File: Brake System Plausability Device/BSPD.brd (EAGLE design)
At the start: 100 x 80 mm, 47 parts, among them IC1 TLC339P, IC2 4081N, IC3 4013N, IC4 4093N, IC5 4013N, IC6 4069N, X1 ERR_STATE_OUT

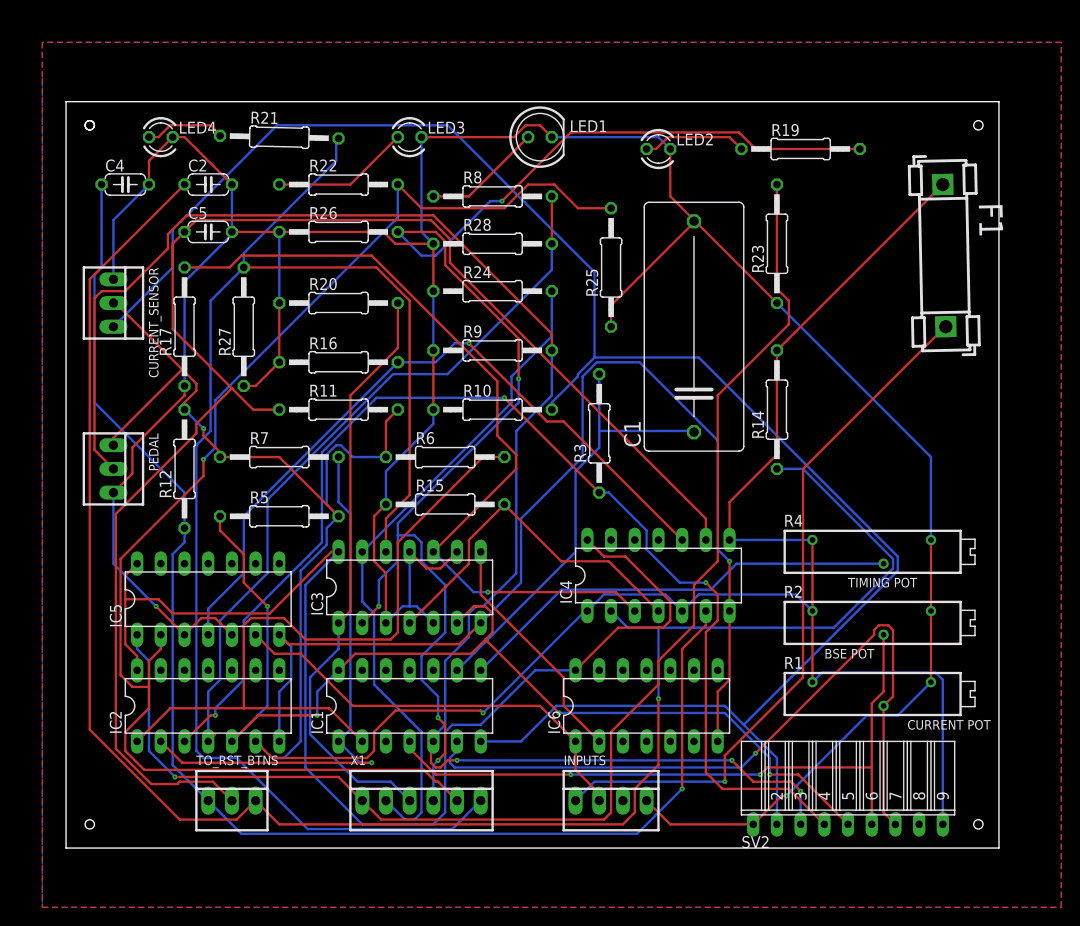
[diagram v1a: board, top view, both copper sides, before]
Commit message: PCB Designs
Rev C
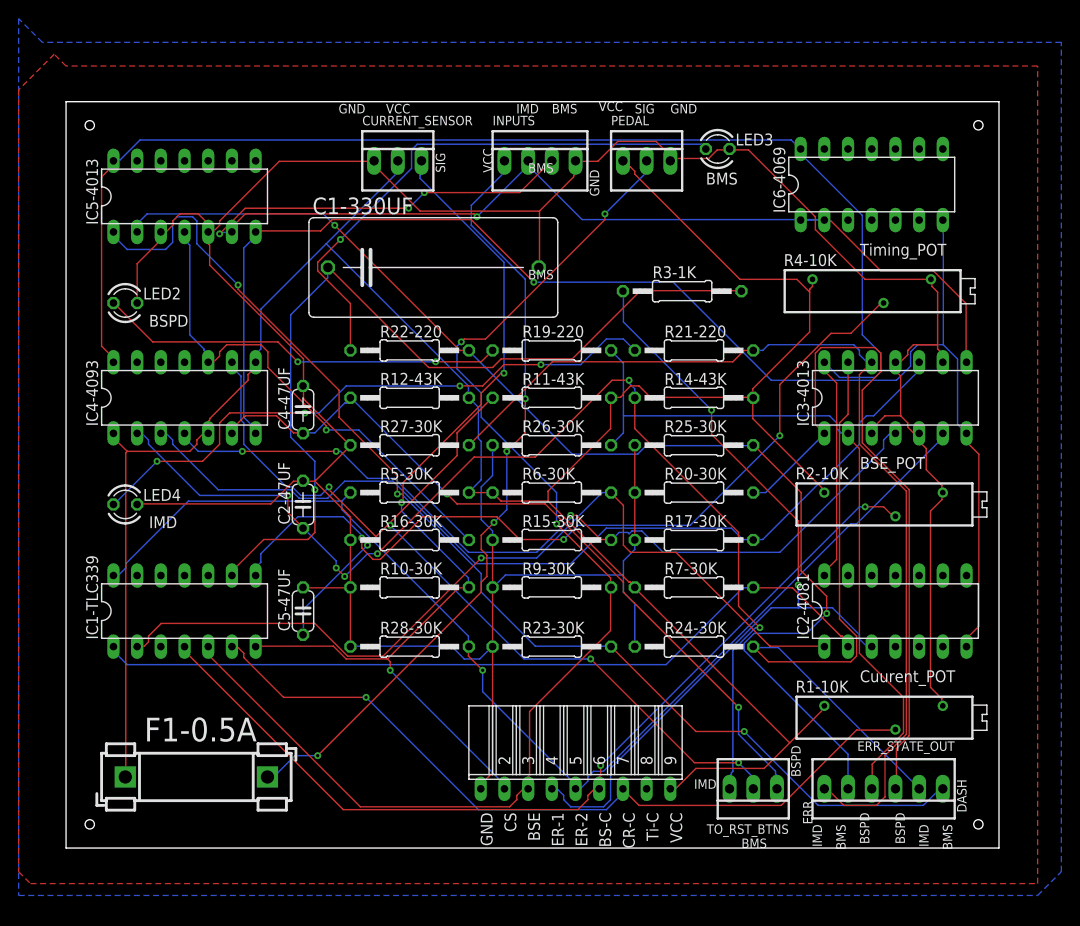
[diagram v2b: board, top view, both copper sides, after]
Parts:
- removed C1: 330u, rcl:C225-108X268
- removed C2, C4, C5: 47uF, rcl:C050-024X044
- removed F1: FUSEBLANK_5X20MM, fuse:FUSE_HOLDER_5X20MM
- removed IC1: TLC339P, linear:DIL14
- removed IC2: 4081N, 40xx:DIL14
- removed IC3, IC5: 4013N, 40xx:DIL14
- removed IC4: 4093N, 40xx:DIL14
- removed IC6: 4069N, 40xx:DIL14
- removed LED1: (no value), led:LED5MM
- removed R1, R2, R4: (no value), rcl:RTRIM3006P
- removed R10, R15, R16, R17, R20, R23, R24, R25, R26, R27, R28, R5, R6, R7, R9: 30k, rcl:0207/12
- removed R11, R12, R14: 43k, rcl:0207/12
- removed R19, R21, R22, R8: 220, rcl:0207/12
- removed R3: 1k, rcl:0207/12
- removed SV2: (no value), con-lsta:FE09W
- removed X1: ERR_STATE_OUT, con-molex:22-23-2061
- added C1-330UF: 330u, rcl:C225-108X268
- added C2-47UF, C4-47UF, C5-47UF: 47uF, rcl:C050-024X044
- added ERR_STATE_OUT: ERR_STATE_OUT, con-molex:22-23-2061
- added F1-0.5A: FUSEBLANK_5X20MM, fuse:FUSE_HOLDER_5X20MM
- added GND: (no value), con-lsta:FE09W
- added IC1-TLC339: TLC339P, linear:DIL14
- added IC2-4081: 4081N, 40xx:DIL14
- added IC3-4013, IC5-4013: 4013N, 40xx:DIL14
- added IC4-4093: 4093N, 40xx:DIL14
- added IC6-4069: 4069N, 40xx:DIL14
- added R1-10K, R2-10K, R4-10K: (no value), rcl:RTRIM3006P
- added R10-30K, R15-30K, R16-30K, R17-30K, R20-30K, R23-30K, R24-30K, R25-30K, R26-30K, R27-30K, R28-30K, R5-30K, R6-30K, R7-30K, R9-30K: 30k, rcl:0207/12
- added R11-43K, R12-43K, R14-43K: 43k, rcl:0207/12
- added R19-220, R21-220, R22-220: 220, rcl:0207/12
- added R3-1K: 1k, rcl:0207/12
- moved INPUTS 69.0 mm to (50.8, 73.7)
- moved PEDAL 66.0 mm to (62.2, 73.7), turned to 0 degrees
- moved LED2 59.5 mm to (6.35, 58.4)
- moved TO_RST_BTNS 55.9 mm to (73.7, 6.35), turned to 180 degrees
- moved LED4 39.6 mm to (6.35, 36.8)
- moved CURRENT_SENSOR 34.1 mm to (35.6, 73.7), turned to 0 degrees
- moved LED3 33.0 mm to (69.8, 74.9)
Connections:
- removed net N$16: IC2.4, R28.2, R8.2
- removed net N$17: LED1.A, R8.1
- net BMS: now also IC5-4013.6
- net BMS_DASH: now also ERR_STATE_OUT.1, IC5-4013.1, R23-30K.2; no longer IC5.1, R23.2, X1.1
- net BMS_ERR: now also ERR_STATE_OUT.5, IC5-4013.2, R22-220.2, R25-30K.2; no longer IC5.2, R22.2, R25.2, X1.5
- net BMS_RST: now also IC4-4093.10, IC5-4013.4, R16-30K.2; no longer IC4.10, IC5.4, R16.2
- net BSE: now also GND.3, IC1-TLC339.5, R9-30K.2; no longer IC1.5, R9.2, SV2.3
- net BSE_POT: now also GND.6, IC1-TLC339.4, R2-10K.2; no longer IC1.4, R2.2, SV2.6
- net BSPD_DASH: now also ERR_STATE_OUT.3, IC3-4013.1, R20-30K.2; no longer IC3.1, R20.2, X1.3
- net BSPD_ERR: now also ERR_STATE_OUT.4, IC3-4013.2, R19-220.2, R26-30K.2; no longer IC3.2, R19.2, R26.2, X1.4
- net BSPD_RST: now also IC3-4013.4, IC4-4093.4, R15-30K.2; no longer IC3.4, IC4.4, R15.2
- net CURRENT_POT: now also GND.7, IC1-TLC339.6, R1-10K.2; no longer IC1.6, R1.2, SV2.7
- net CURRENT_SENSOR: now also GND.2, IC1-TLC339.7, R10-30K.2; no longer IC1.7, R10.2, SV2.2
- net ERROR_1: now also GND.4, IC2-4081.3, R3-1K.1; no longer IC2.3, R3.1, SV2.4
- net ERROR_2: now also GND.5, IC1-TLC339.14, IC3-4013.6, R28-30K.2, R5-30K.1; no longer IC1.14, IC2.5, IC3.6, R5.1, SV2.5
- net ESO_BMS_RST: now also C5-47UF.1, IC4-4093.9, R11-43K.1; no longer C5.1, IC4.9, R11.1
- net ESO_BSPD_RST: now also C4-47UF.1, IC4-4093.6, R12-43K.1; no longer C4.1, IC4.6, R12.1
- net ESO_IMD_RST: now also C2-47UF.1, IC4-4093.2, R14-43K.1; no longer C2.1, IC4.2, R14.1
- net GND: now also C1-330UF.2, C2-47UF.2, C4-47UF.2, C5-47UF.2, GND.1, IC3-4013.11, IC3-4013.3, IC3-4013.5, IC3-4013.9, IC5-4013.3, IC5-4013.5, R1-10K.3, R10-30K.1, R15-30K.1, R16-30K.1, R17-30K.1, R2-10K.3, R20-30K.1, R23-30K.1, R24-30K.1, R25-30K.1, R26-30K.1, R27-30K.1, R28-30K.1, R4-10K.3, R9-30K.1; no longer C1.2, C2.2, C4.2, C5.2, IC3.11, IC3.3, IC3.5, IC3.9, IC5.3, IC5.5, LED1.K, R1.3, R10.1, R15.1, R16.1, R17.1, R2.3, R20.1, R23.1, R24.1, R25.1, R26.1, R27.1, R28.1, R4.3, R9.1, SV2.1
- net IMD: now also IC6-4069.1; no longer IC5.6, IC6.1
- net IMD_DASH: now also ERR_STATE_OUT.2, IC3-4013.13, R24-30K.2; no longer IC3.13, R24.2, X1.2
- net IMD_ERR: now also ERR_STATE_OUT.6, IC3-4013.12, R21-220.2, R27-30K.2; no longer IC3.12, R21.2, R27.2, X1.6
- net IMD_RST: now also IC3-4013.10, IC4-4093.3, R17-30K.2; no longer IC3.10, IC4.3, R17.2
- net N$1: now also IC1-TLC339.2, IC2-4081.1, R6-30K.2; no longer IC1.2, IC2.1, R6.2
- net N$15: now also R21-220.1; no longer R21.1
- net N$2: now also IC1-TLC339.1, IC2-4081.2, R7-30K.2; no longer IC1.1, IC2.2, R7.2
- net N$21: now also R19-220.1; no longer R19.1
- net N$4: now also F1-0.5A.2; no longer F1.2
- net N$5: now also IC3-4013.8, IC6-4069.2; no longer IC3.8, IC6.2
- net N$6: now also C1-330UF.1, IC1-TLC339.9, R3-1K.2; no longer C1.1, IC1.9, R3.2
- net N$9: now also R22-220.1; no longer R22.1
- net TIMED_POT: now also IC1-TLC339.8, R4-10K.2; no longer IC1.8, R4.2
- net TIME_POT: now also GND.8; no longer SV2.8
- net V+: now also IC1-TLC339.3; no longer IC1.3
- net V-: now also IC1-TLC339.12; no longer IC1.12
- net VCC: now also F1-0.5A.1, GND.9, IC4-4093.1, IC4-4093.5, IC4-4093.8, R1-10K.1, R11-43K.2, R12-43K.2, R14-43K.2, R2-10K.1, R4-10K.1, R5-30K.2, R6-30K.1, R7-30K.1; no longer F1.1, IC2.6, IC4.1, IC4.5, IC4.8, R1.1, R11.2, R12.2, R14.2, R2.1, R4.1, R5.2, R6.1, R7.1, SV2.9
- net VDD: now also IC2-4081.14, IC3-4013.14, IC4-4093.14, IC5-4013.14, IC6-4069.14; no longer IC2.14, IC3.14, IC4.14, IC5.14, IC6.14
- net VSS: now also IC2-4081.7, IC3-4013.7, IC4-4093.7, IC5-4013.7, IC6-4069.7; no longer IC2.7, IC3.7, IC4.7, IC5.7, IC6.7
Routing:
- net CURRENT_SENSOR: track 195.0 -> 102.9 mm, vias 0 -> 3
- net ESO_IMD_RST: track 199.4 -> 121.0 mm, vias 1 -> 6
- net N$16: track 78.2 -> 0.00 mm
- net BSPD_ERR: track 147.6 -> 78.5 mm, vias 5 -> 0
- net ESO_BSPD_RST: track 146.8 -> 82.6 mm, vias 1 -> 2
- net N$15: track 8.68 -> 65.1 mm, vias 0 -> 4
- net BSPD_RST: track 38.2 -> 92.0 mm, vias 0 -> 3
- net IMD_ERR: track 154.5 -> 106.5 mm
- net N$6: track 48.3 -> 94.4 mm, vias 0 -> 1
- net N$9: track 14.8 -> 59.1 mm, vias 0 -> 1
- net BSE: track 174.8 -> 130.6 mm
- net ESO_BMS_RST: track 158.1 -> 114.0 mm, vias 0 -> 5
- net TIMED_POT: track 47.9 -> 90.3 mm, vias 0 -> 3
- net BMS: track 0.00 -> 40.2 mm, vias 0 -> 3
- net ERROR_1: track 126.7 -> 89.9 mm, vias 3 -> 2
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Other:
- board text added: "BMS"
- board text added: "BS-C"
- board text added: "BSE"
- board text added: "BSE_POT"
- board text added: "BSPD"
- board text added: "CR-C"
- board text added: "CS"
- board text added: "Cuurent_POT"
- board text added: "DASH"
- board text added: "ER-1"
- board text added: "ER-2"
- board text added: "ERR"
- board text added: "GND"
- board text added: "IMD"
- board text added: "SIG"
- board text added: "Ti-C"
- board text added: "Timing_POT"
- board text added: "VCC"
- board text removed: "BSE POT"
- board text removed: "CURRENT POT"
- board text removed: "TIMING POT"
